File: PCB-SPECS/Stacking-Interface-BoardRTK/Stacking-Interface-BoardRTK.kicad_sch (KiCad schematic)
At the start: 15 parts

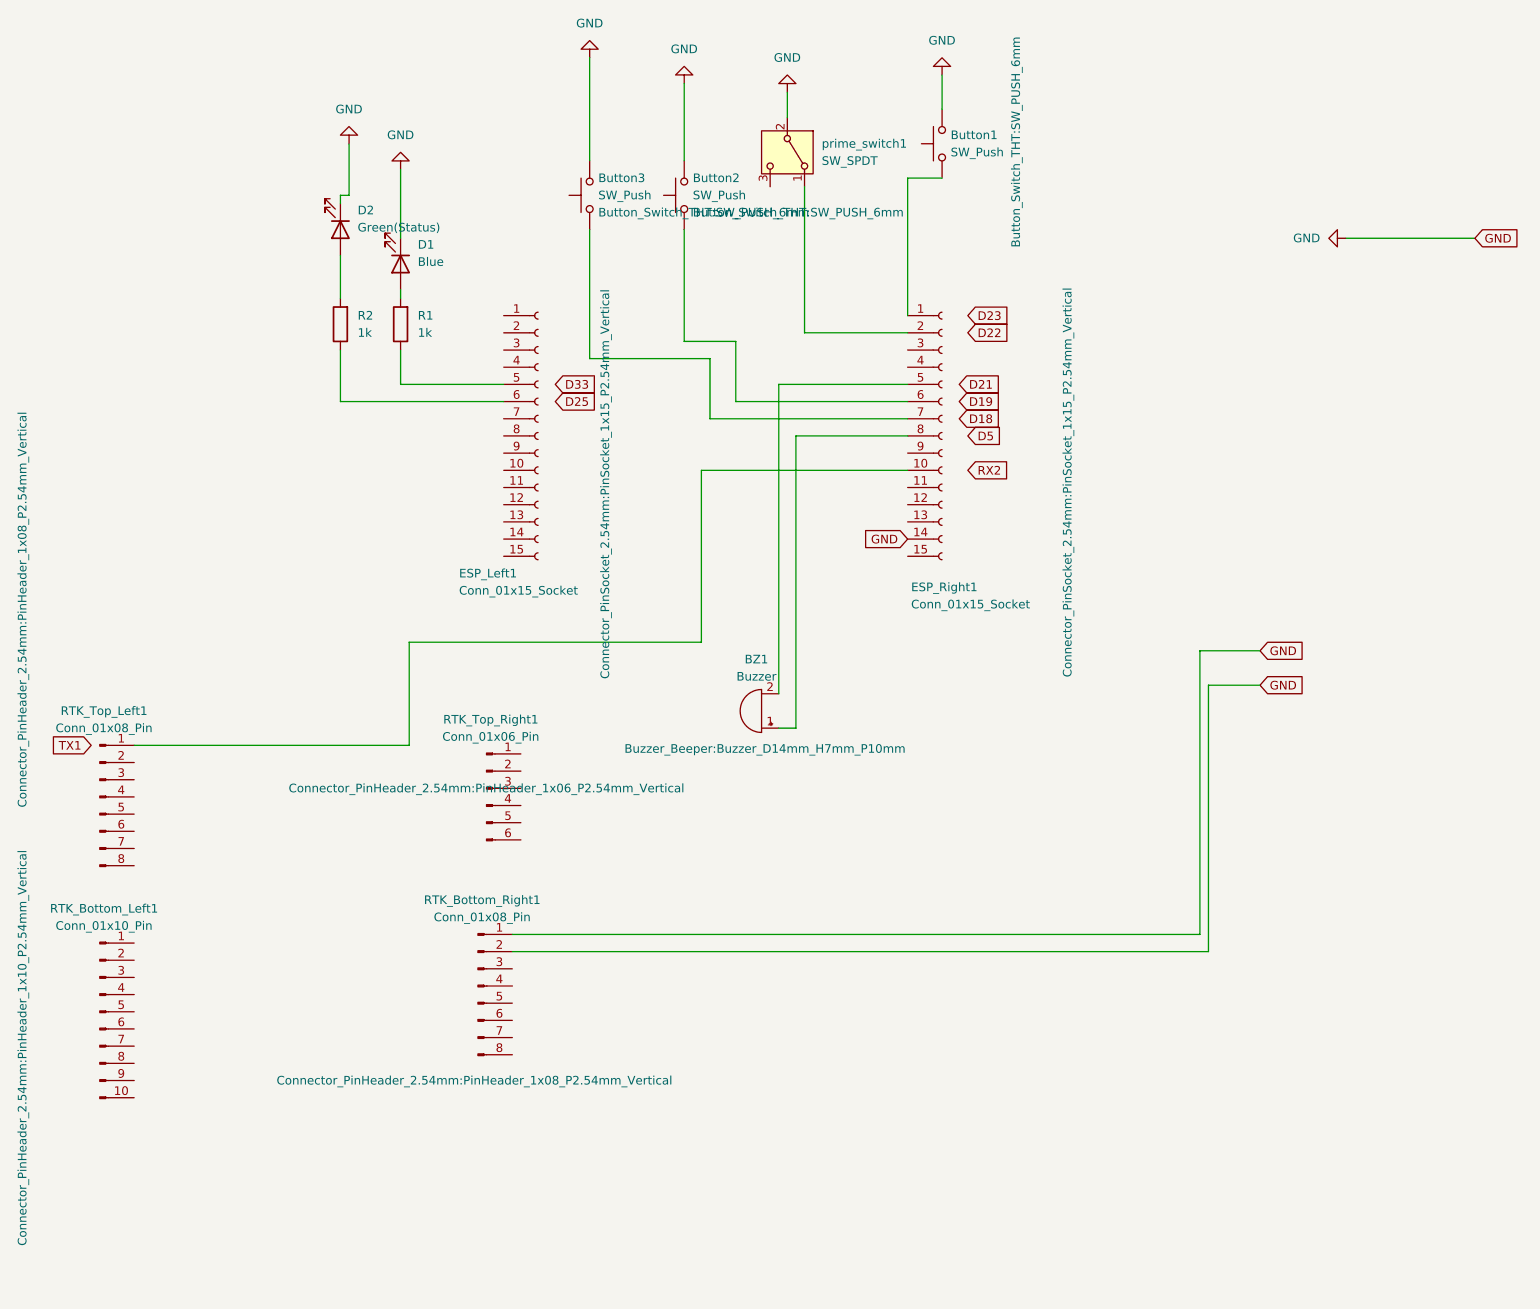
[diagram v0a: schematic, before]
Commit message: finished designing pcb
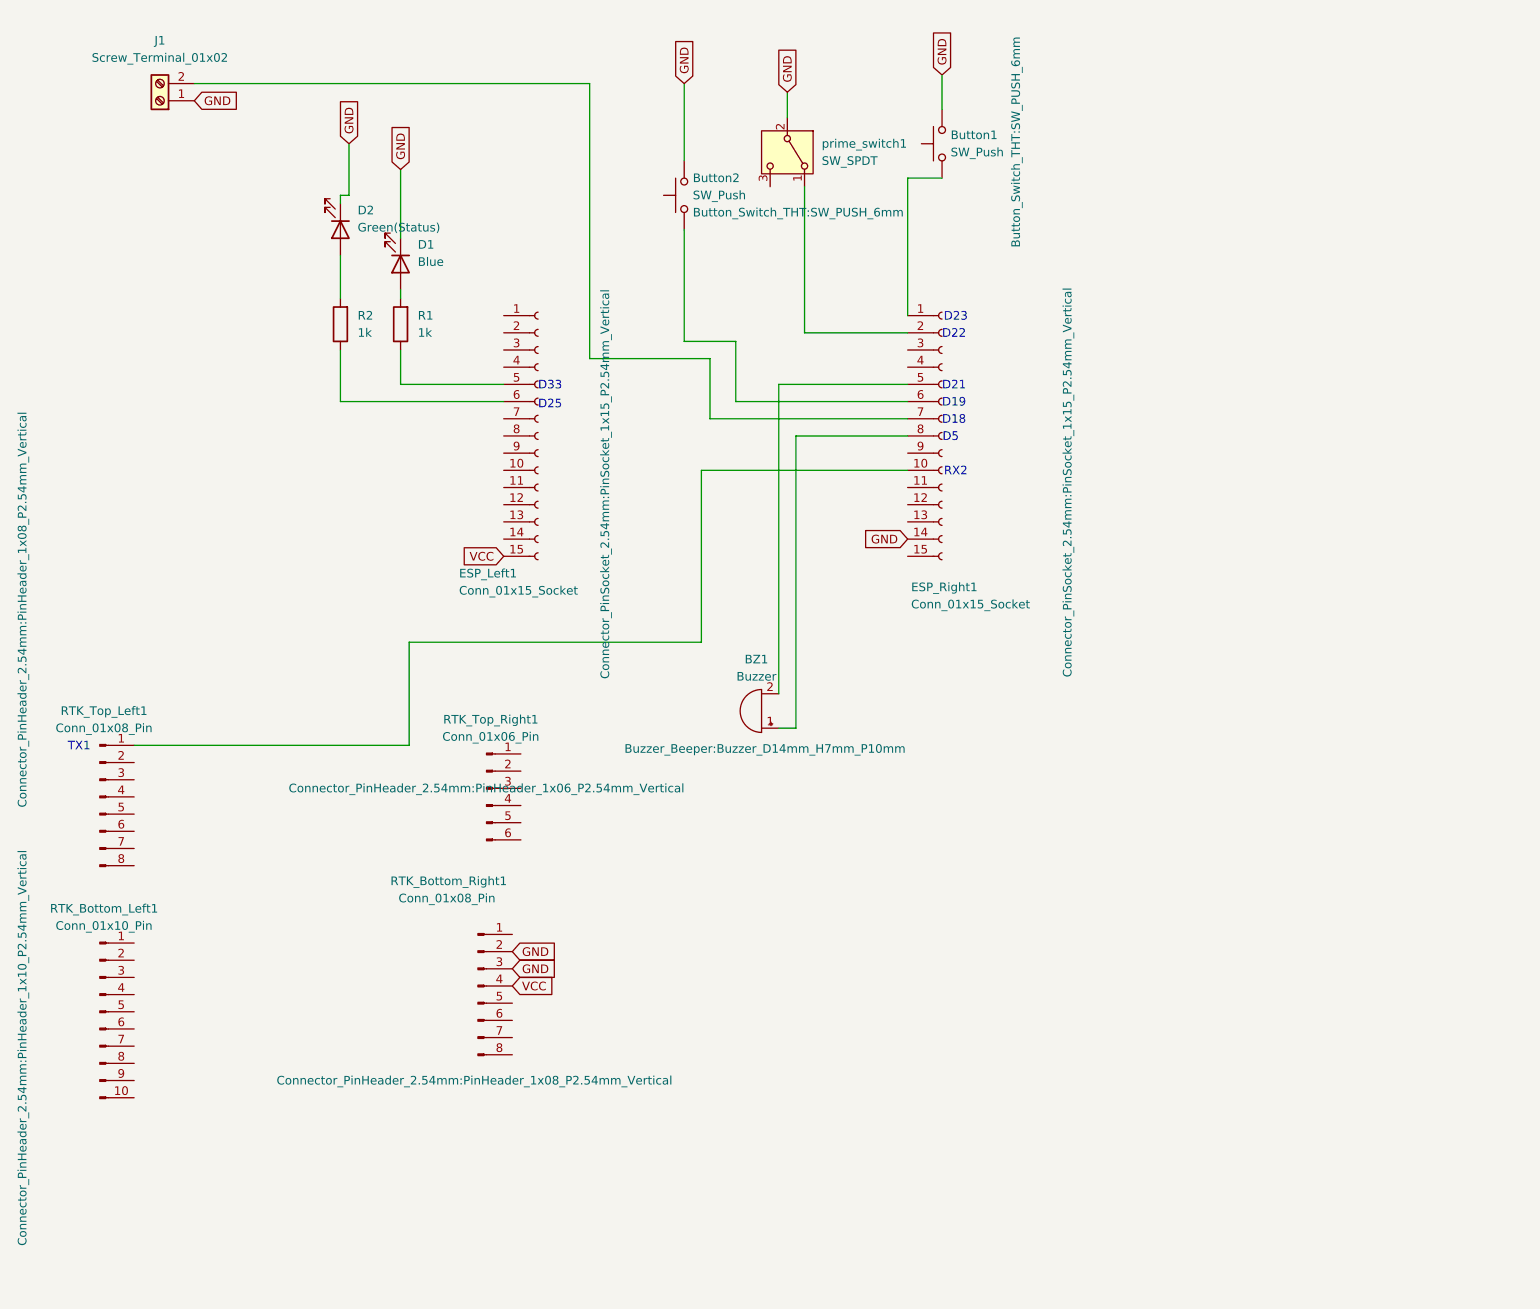
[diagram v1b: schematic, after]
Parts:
- removed Button3: SW_Push, Button_Switch_THT:SW_PUSH_6mm, symbol Switch:SW_Push
- added J1: Screw_Terminal_01x02, TerminalBlock:TerminalBlock_Altech_AK300-2_P5.00mm, symbol Connector:Screw_Terminal_01x02
- prime_switch1: footprint Button_Switch_THT:SW_Slide-03_Wuerth-WS-SLTV_10x2.5x6.4_P2.54mm -> watermelonstuff:spdt_switch
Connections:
- net GND: now also RTK_Bottom_Right1.3 (Pin_3), J1.1 (Pin_1); no longer RTK_Bottom_Right1.1 (Pin_1)
- net at ESP_Right1.7 (Pin_7): now also J1.2 (Pin_2)
- net VCC: now reaches ESP_Left1.15 (Pin_15)
- net VCC: now also RTK_Bottom_Right1.4 (Pin_4)
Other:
- note added: "D18"
- note added: "D19"
- note added: "D21"
- note added: "D22"
- note added: "D23"
- note added: "D25"
- note added: "D33"
- note added: "D5"
- note added: "RX2"
- note added: "TX1"
